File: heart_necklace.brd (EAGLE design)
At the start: 33.9 x 31.6 mm, 23 parts, among them SW1 300mA/4V

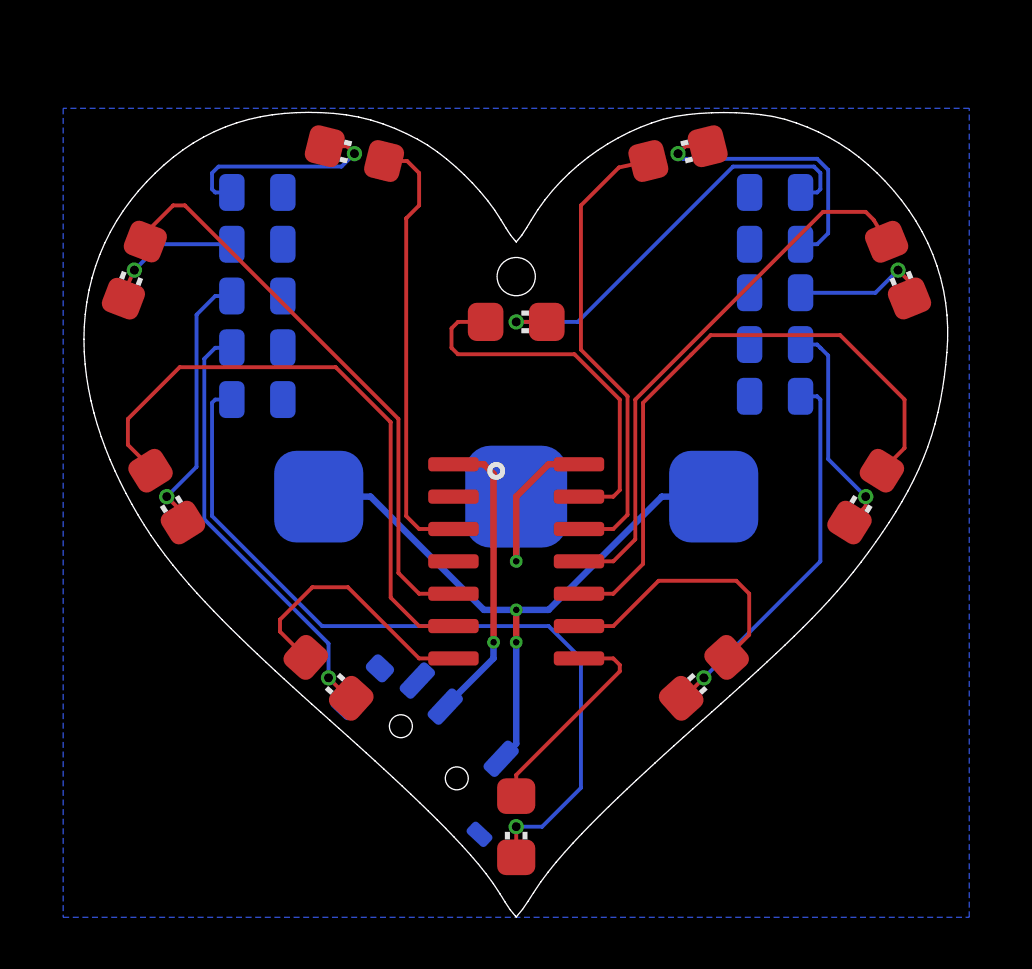
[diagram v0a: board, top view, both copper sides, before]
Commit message: changes
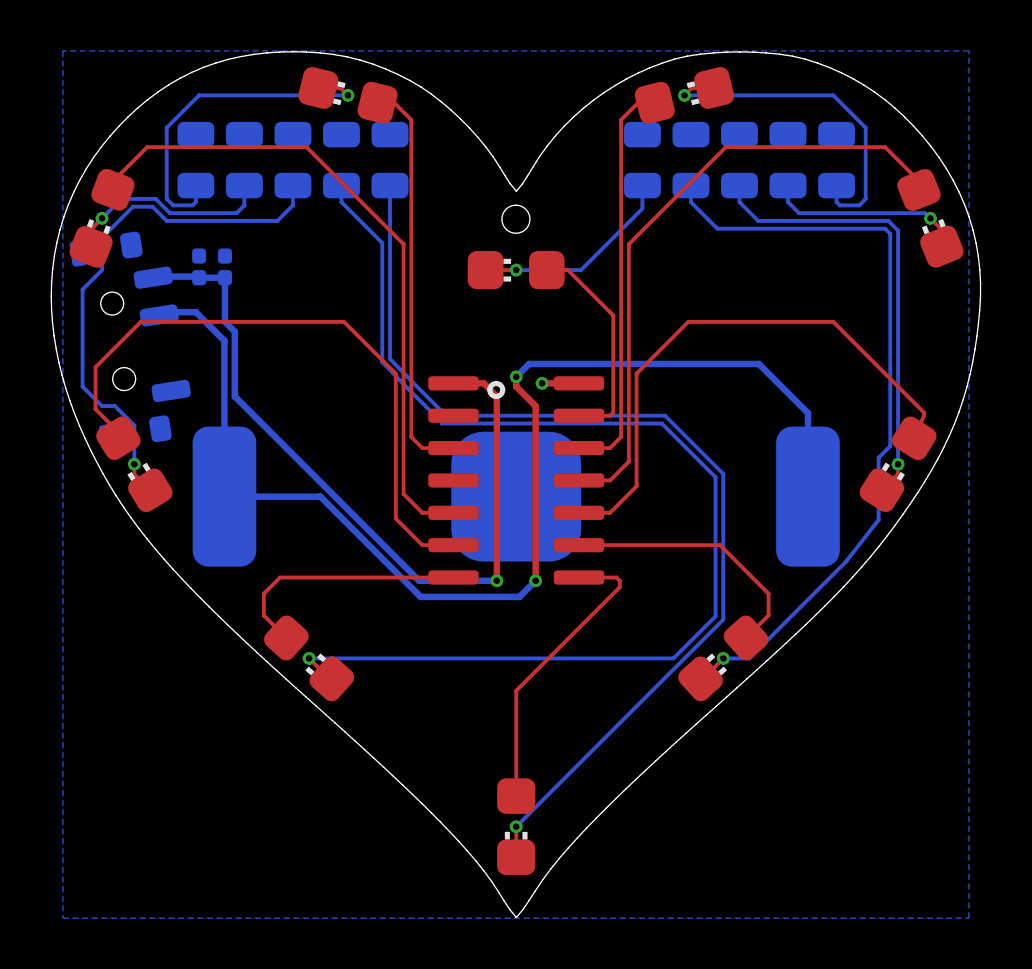
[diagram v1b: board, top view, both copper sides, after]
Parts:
- removed BATT2: BR-1225/3V/48mAh, PiB_batteries:BR-1225
- added BATT1: (no value), PiB_batteries:CR-2032
- added C1, C2: 10uF/10V, PiB_capacitors:_CER_SMD_0402
- MCU1: value ATTINY84 -> ATTiny84
- moved SW1 20.2 mm to (-15.6, 22.6), turned to 171 degrees
- moved R6 10.7 mm to (-4.95, 29.7), turned to 270 degrees
- moved R5 9.84 mm to (6.86, 29.7), turned to 270 degrees
- moved R7 8.07 mm to (-6.86, 29.7), turned to 270 degrees
- moved R4 7.37 mm to (8.76, 29.7), turned to 270 degrees
- moved R8 5.51 mm to (-8.76, 29.7), turned to 270 degrees
- moved R1 5.36 mm to (4.95, 29.7), turned to 270 degrees
- moved R3 5.23 mm to (10.7, 29.7), turned to 270 degrees
- moved R2 4.09 mm to (12.6, 29.7), turned to 270 degrees
- moved R9 3.34 mm to (-10.7, 29.7), turned to 270 degrees
- moved MCU1 3.17 mm to (0.00, 17.1)
- moved R10 2.73 mm to (-12.6, 29.7), turned to 270 degrees
- moved LED3 2.40 mm to (16.3, 27.4)
- moved LED9 2.40 mm to (-16.3, 27.4)
- moved LED10 2.30 mm to (-6.60, 32.3)
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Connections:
- net GND: now also BATT1.-, C1.2, C2.2; no longer BATT2.-
- net N$11: now also C1.1, C2.1, SW1.3; no longer SW1.2
- net VBATT: now also BATT1.+_1, BATT1.+_2, SW1.2; no longer BATT2.+_1, BATT2.+_2, SW1.1
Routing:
- net N$7: track 17.0 -> 45.9 mm
- net VBATT: track 25.3 -> 47.4 mm
- net N$11: track 11.6 -> 30.1 mm
- net N$5: track 14.9 -> 30.1 mm
- net N$8: track 10.6 -> 20.9 mm
- net N$1: track 17.2 -> 8.06 mm
- net N$4: track 8.69 -> 17.8 mm
- net N$6: track 31.5 -> 40.2 mm
- net GND: track 8.07 -> 1.45 mm
- net LED2: track 14.9 -> 8.56 mm
- net N$9: track 8.65 -> 13.7 mm
- net LED4: track 8.54 -> 11.8 mm
- net LED1: track 22.7 -> 25.9 mm
- net LED5: track 24.9 -> 21.8 mm
- net LED3: track 21.6 -> 24.7 mm
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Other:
- board size 33.9 x 31.6 mm -> 36.5 x 34 mm
- board text added: "Rev 2"
- board text removed: "Rev 1"
